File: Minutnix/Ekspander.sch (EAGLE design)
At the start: 9 parts

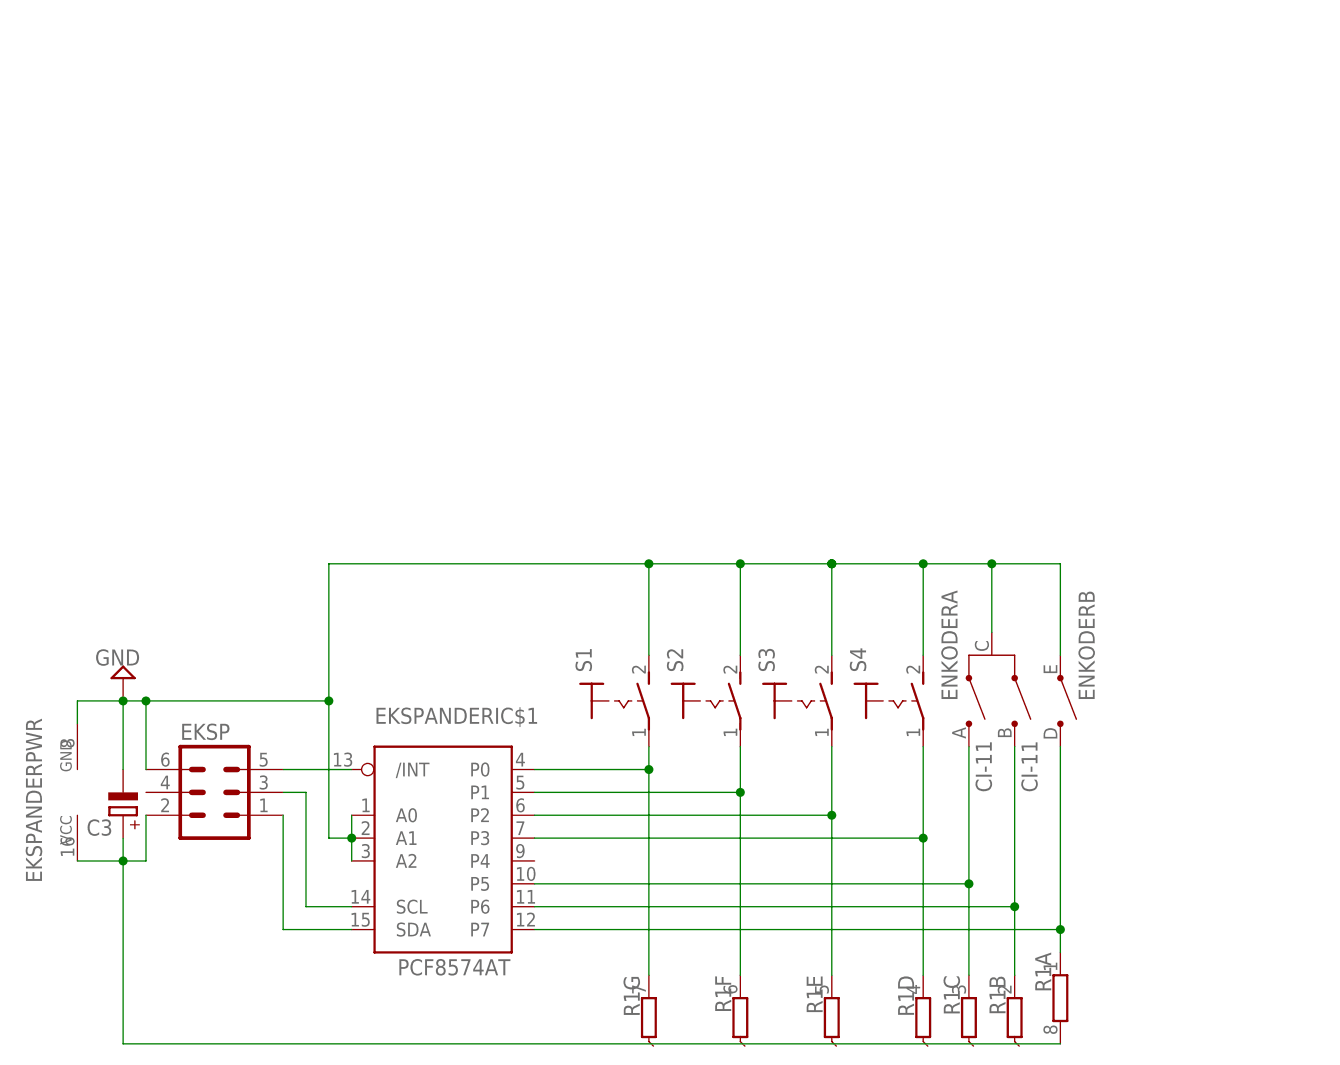
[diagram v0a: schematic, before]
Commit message: Archivisation and actualisation
Archivisation of 1 version of boards
New version of boards
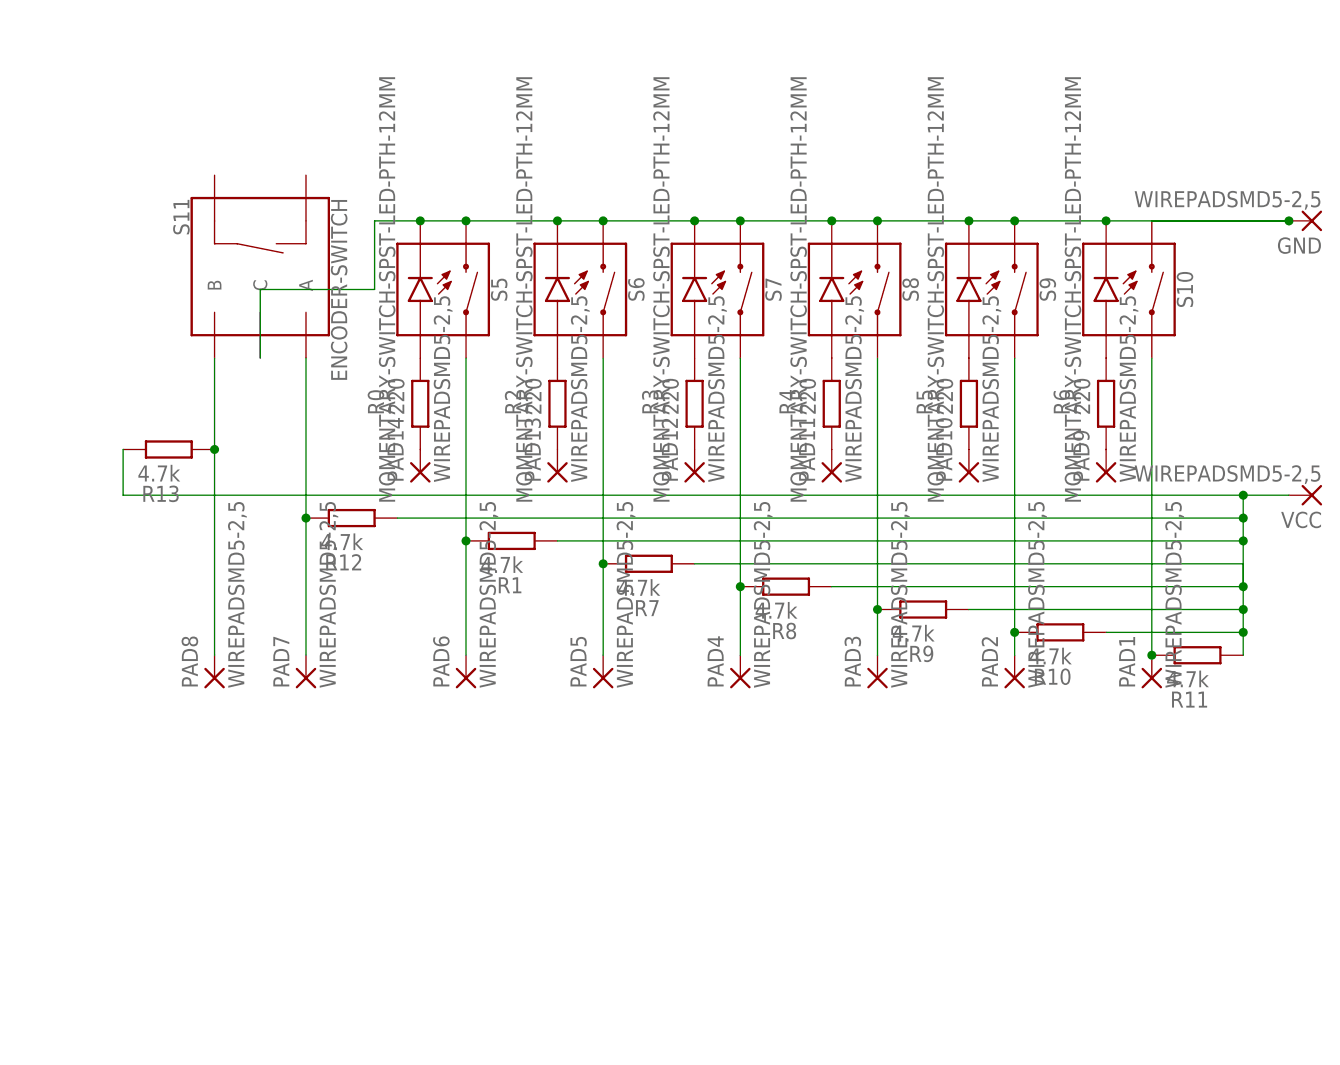
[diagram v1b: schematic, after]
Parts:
- removed C3: (no value), rcl:CPOL-EU140CLH-1010
- removed EKSP: (no value), con-harting-ml:ML6
- removed EKSPANDER: PCF8574AT, i2c:PCF8574AT
- removed ENKODER: CI-11, piher:CI-11
- removed S1, S2, S3, S4: (no value), switch:MS243
- added GND, PAD1, PAD10, PAD11, PAD12, PAD13, PAD14, PAD2, PAD3, PAD4, PAD5, PAD6, PAD7, PAD8, PAD9, VCC: WIREPADSMD5-2,5, wirepad:WIREPADSMD5-2,5
- added R0, R2, R3, R4, R5, R6: 220, rcl:R-EU_01005
- added R10, R11, R12, R13, R7, R8, R9: 4.7k, rcl:R-EU_01005
- added S10, S5, S6, S7, S8, S9: MOMENTARY-SWITCH-SPST-LED-PTH-12MM, SparkFun-Switches:MOMENTARY-SWITCH-SPST-LED-PTH-12MM
- added S11: ENCODER-SWITCH, SparkFun-Switches:ENCODER-SWITCH
- R1: value (none) -> 4.7k; device resistor-bourns:2NBS08-7E -> rcl:R-EU_01005
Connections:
- removed net GND: C3.-, EKSP.6, EKSPANDERIC$1.A0, EKSPANDERIC$1.A1, EKSPANDERIC$1.A2, EKSPANDERPWR.GND, ENKODERA.C, ENKODERB.E, S1.S, S2.S, S3.S, S4.S
- new net N$12: PAD14.P, R0.1
- new net N$13: PAD1.P, R11.2, S10.1
- new net N$14: PAD8.P, R13.1, S11.B
- new net N$15: PAD7.P, R12.2, S11.A
- new net N$16: PAD6.P, R1.2, S5.1
- new net N$17: PAD5.P, R7.2, S6.1
- new net N$18: PAD4.P, R8.2, S7.1
- new net N$19: PAD3.P, R9.2, S8.1
- new net N$20: PAD2.P, R10.2, S9.1
- new net N$21: R1.1, R10.1, R11.1, R12.1, R13.2, R7.1, R8.1, R9.1, VCC.P
- new net N$85: GND.P, S10.2, S10.C, S11.C, S5.2, S5.C, S6.2, S6.C, S7.2, S7.C, S8.2, S8.C, S9.2, S9.C
- net N$1: now also R0.2, S5.A; no longer EKSP.5, EKSPANDERIC$1./INT
- net N$10: now also PAD12.P, R3.1; no longer EKSPANDERIC$1.P1, R1F.1, S2.P
- net N$11: now also PAD13.P, R2.1; no longer EKSPANDERIC$1.P0, R1G.1, S1.P
- net N$2: now also R2.2, S6.A; no longer EKSP.1, EKSPANDERIC$1.SDA
- net N$3: now also R3.2, S7.A; no longer EKSP.3, EKSPANDERIC$1.SCL
- net N$4: now also R4.2, S8.A; no longer C3.+, EKSP.2, EKSPANDERPWR.VCC, R1A.2
- net N$5: now also R5.2, S9.A; no longer EKSPANDERIC$1.P7, ENKODERB.D, R1A.1
- net N$6: now also R6.2, S10.A; no longer EKSPANDERIC$1.P6, ENKODERA.B, R1B.1
- net N$7: now also PAD9.P, R6.1; no longer EKSPANDERIC$1.P5, ENKODERA.A, R1C.1
- net N$8: now also PAD10.P, R5.1; no longer EKSPANDERIC$1.P3, R1D.1, S4.P
- net N$9: now also PAD11.P, R4.1; no longer EKSPANDERIC$1.P2, R1E.1, S3.P
